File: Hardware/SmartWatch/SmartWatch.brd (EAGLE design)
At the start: 36.8 x 40.6 mm, 73 parts, among them U1 STM32L476, U3 UG-2828GDEDF11, U4 FAN5331SX, U5 APDS-9960, U6 MCP73831, U7 AP2112K-3.3TRG-1

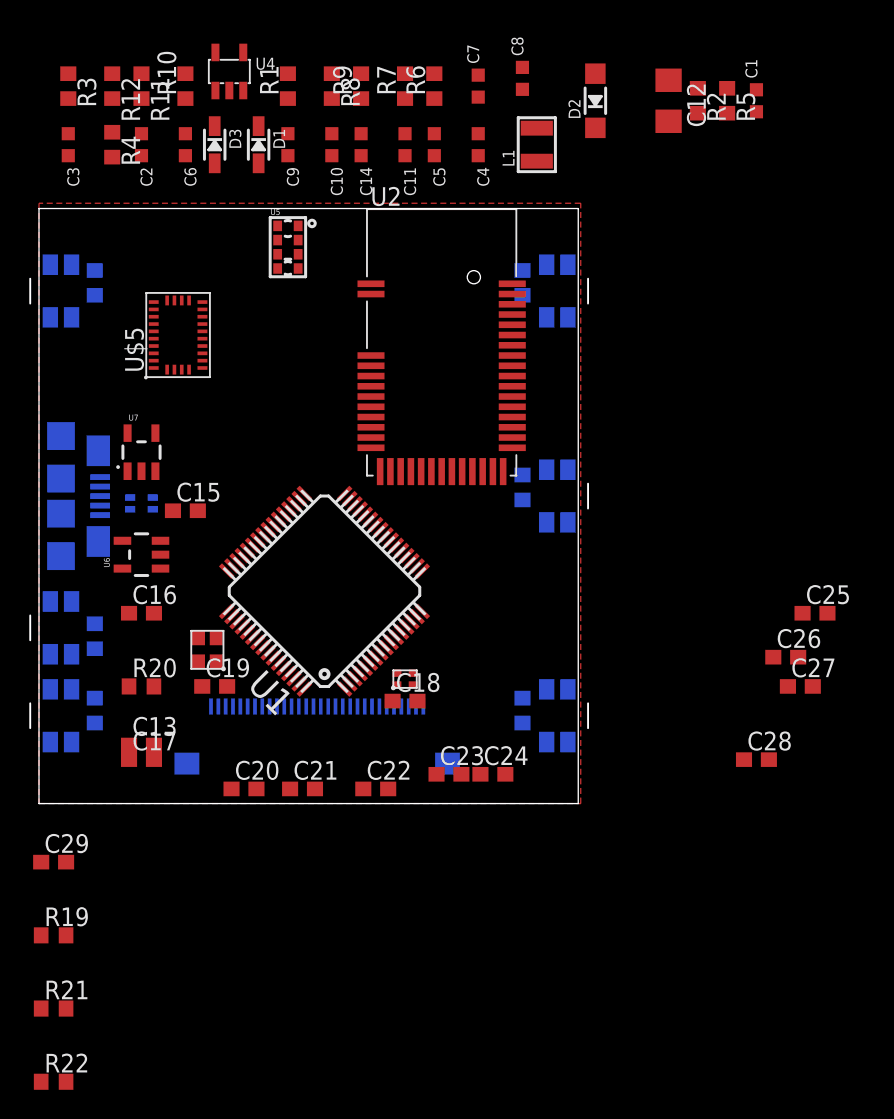
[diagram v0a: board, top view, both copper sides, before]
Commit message: started board layout
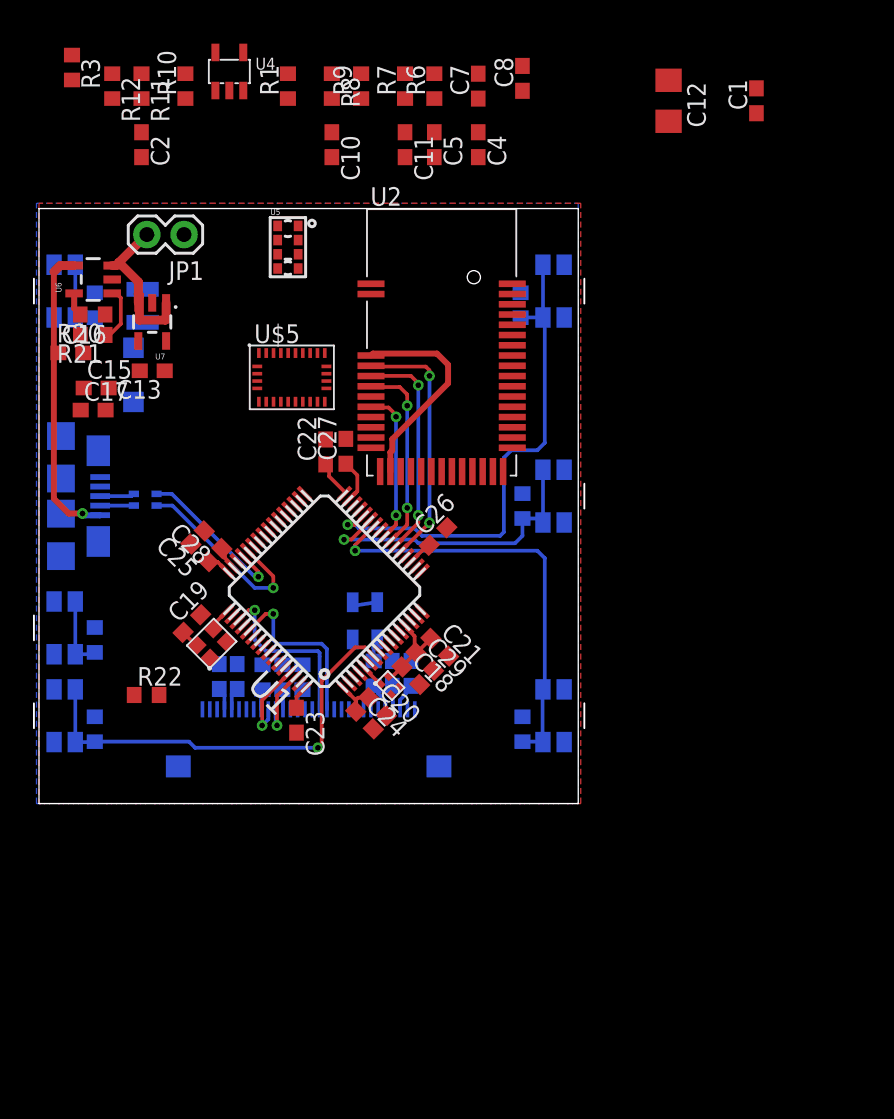
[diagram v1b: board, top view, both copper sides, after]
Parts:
- added JP1: (no value), SparkFun-Connectors:1X02
- C1, C10, C11, C14, C2, C3, C4, C5, C6, C7, C8, C9: device microbuilder:0603-MINI -> resistor:C0603
- moved R2 47.7 mm to (18.0, 8.63), flipped to the bottom
- moved R21 46.1 mm to (3.67, 32.0), turned to 180 degrees
- moved R5 46.0 mm to (22.9, 8.89), flipped to the bottom
- moved C3 42.4 mm to (24.1, 8.89), flipped to the bottom
- moved C25 42.2 mm to (11.0, 17.1), turned to 135 degrees
- moved C28 40.0 mm to (11.9, 18.0), turned to 135 degrees
- moved C6 39.3 mm to (25.4, 8.89), flipped to the bottom, turned to 90 degrees
- moved R4 37.8 mm to (15.3, 8.63), flipped to the bottom
- moved C14 37.3 mm to (13.5, 8.68), flipped to the bottom
- moved D2 36.7 mm to (6.45, 29.3), flipped to the bottom
- moved C9 36.6 mm to (12.3, 8.68), flipped to the bottom
- moved C27 35.0 mm to (21.0, 24.1), turned to 90 degrees
- moved D3 33.9 mm to (21.4, 12.5), flipped to the bottom, turned to 90 degrees
- moved D1 33.5 mm to (23.1, 12.5), flipped to the bottom
- moved L1 29.1 mm to (7.08, 34.0), flipped to the bottom, turned to 270 degrees
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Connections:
- removed net 3.3V: BTN_BACK.3, BTN_BACK.4, BTN_BOOT0.3, BTN_BOOT0.4, BTN_DN.3, BTN_DN.4, BTN_NRST.3, BTN_NRST.4, BTN_SEL.3, BTN_SEL.4, BTN_UP.3, BTN_UP.4, C10.2, C11.2, C12.1, C13.1, C18.1, C19.1, C20.1, C21.1, C22.1, C23.1, C24.1, C25.1, C26.1, C29.1, C3.2, C5.2, C7.1, C9.2, L1.P$1, R21.2, R3.2, R8.2, R9.2, U$39.4, U$41.4, U$5.28, U$5.3, U$5.4, U1.1, U1.13, U1.19, U1.32, U1.48, U1.64, U3.P$27, U3.P$4, U4.4, U4.5, U5.5, U5.8, U7.5
- net +3V3: now also BTN_BACK.3, BTN_BACK.4, BTN_BOOT0.3, BTN_BOOT0.4, BTN_DN.3, BTN_DN.4, BTN_NRST.3, BTN_NRST.4, BTN_SEL.3, BTN_SEL.4, BTN_UP.3, BTN_UP.4, C10.2, C11.2, C12.1, C13.1, C18.1, C19.1, C20.1, C21.1, C22.1, C23.1, C24.1, C25.1, C26.1, C29.1, C3.2, C5.2, C7.1, C9.2, L1.P$1, R21.2, R3.2, R8.2, R9.2, U$39.4, U$41.4, U$5.28, U$5.3, U$5.4, U1.1, U1.13, U1.19, U1.32, U1.48, U1.64, U3.P$27, U3.P$4, U4.4, U4.5, U5.5, U5.8, U7.5
- net GND: now also JP1.1
- net VBAT: now also JP1.2
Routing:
- net +3V3: track 0.00 -> 35.0 mm
- net BTN_UP: track 0.00 -> 34.6 mm, vias 0 -> 1
- net BTN_NRST: track 0.00 -> 30.0 mm, vias 0 -> 1
- net BTN_DN: track 0.00 -> 29.5 mm, vias 0 -> 1
- net BTN_SEL: track 0.00 -> 21.3 mm, vias 0 -> 1
- net VUSB: track 0.00 -> 21.0 mm, vias 0 -> 1
- net BT_SCK: track 0.00 -> 17.2 mm, vias 0 -> 2
- net BT_MISO: track 0.00 -> 15.1 mm, vias 0 -> 2
- net D-: track 0.00 -> 13.6 mm, vias 0 -> 1
- net BT_MOSI: track 0.00 -> 13.1 mm, vias 0 -> 2
- net OLED_SCK: track 0.00 -> 12.2 mm, vias 0 -> 1
- net OLED_MOSI: track 0.00 -> 12.1 mm, vias 0 -> 1
- net VBAT: track 0.00 -> 11.3 mm
- net D+: track 0.00 -> 11.2 mm, vias 0 -> 1
- net BT_INT: track 0.00 -> 10.4 mm, vias 0 -> 2
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- added copper zone on layer 16, net GND
